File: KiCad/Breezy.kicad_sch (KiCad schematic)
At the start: 18 parts, among them J1 Line Voltage Input 120VAC / 6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, J2 Line Voltage Output 120VAC / 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, K1 5V, Q1 2N3904

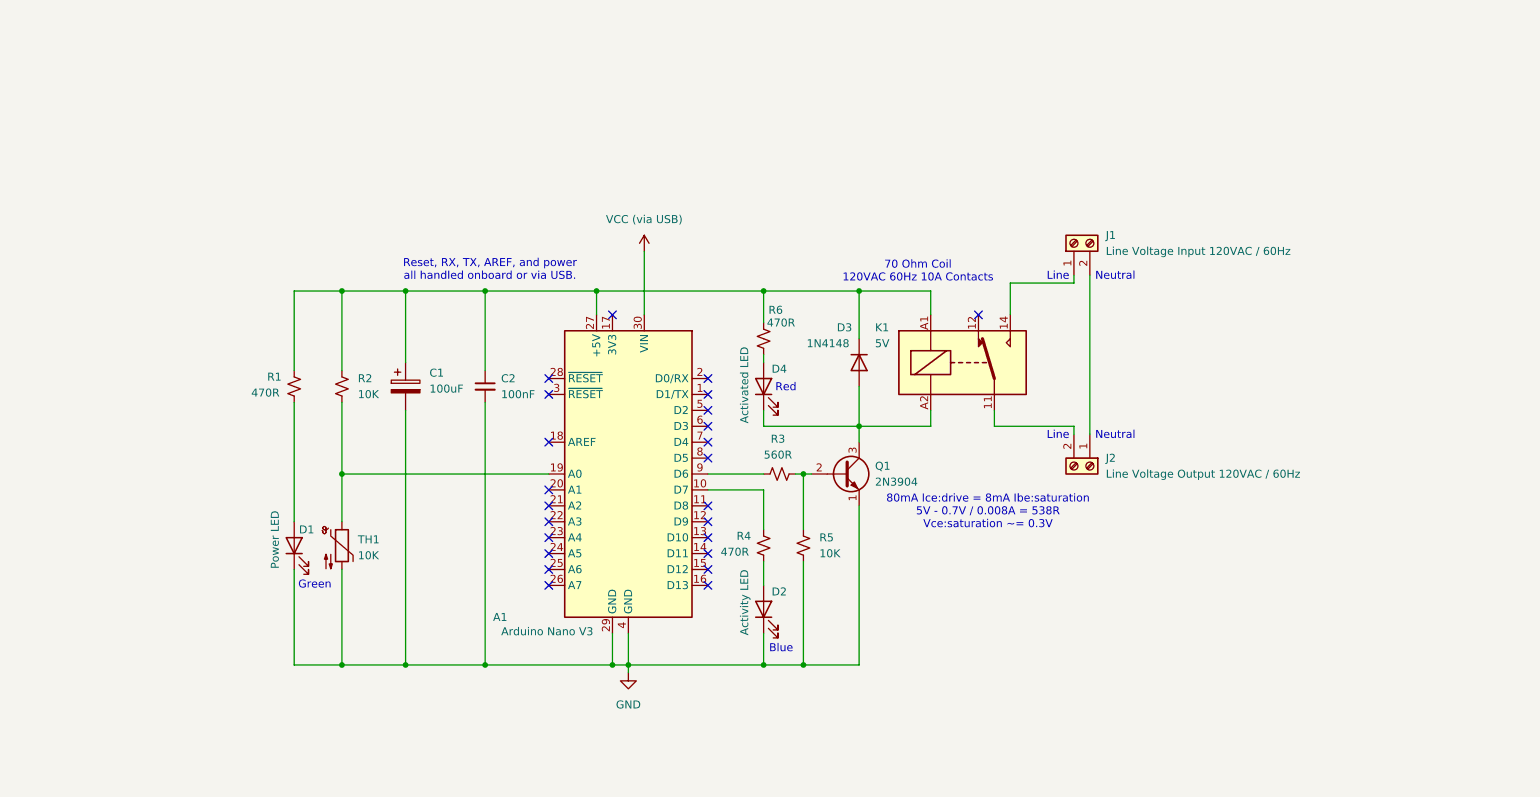
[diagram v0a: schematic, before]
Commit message: Update Breezy
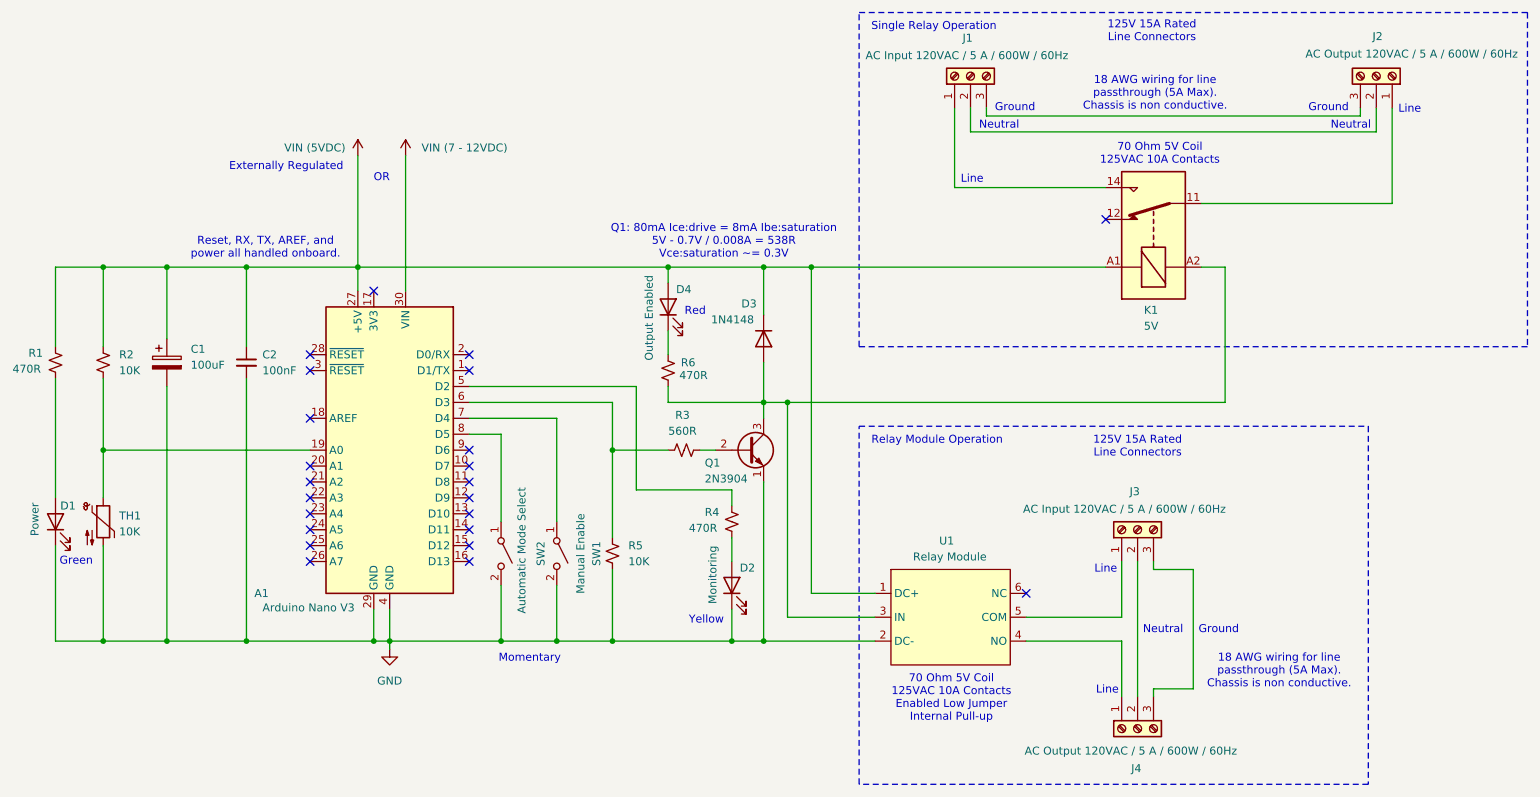
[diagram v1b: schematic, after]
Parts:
- removed J1: Line Voltage Input 120VAC / 60Hz, symbol Connector:Screw_Terminal_01x02
- removed J2: Line Voltage Output 120VAC / 60Hz, symbol Connector:Screw_Terminal_01x02
- added J1, J3: AC Input 120VAC / 5 A / 600W / 60Hz, symbol Connector:Screw_Terminal_01x03
- added J2, J4: AC Output 120VAC / 5 A / 600W / 60Hz, symbol Connector:Screw_Terminal_01x03
- added SW1: Manual Enable, symbol Switch:SW_SPST
- added SW2: Automatic Mode Select, symbol Switch:SW_SPST
- added U1: ~, symbol Custom:Relay Module
- D1: value Power LED -> Power
- D2: value Activity LED -> Monitoring
- D4: value Activated LED -> Output Enabled
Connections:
- net GND: now also SW1.2 (B), SW2.2 (B), U1.2 (DC-)
- net VIN (5VDC): now reaches A1.27 (+5V), C1.1, C2.1, D3.1 (K), K1.A1, R1.1, R2.1
- net VIN (5VDC): now also D4.2 (A), U1.1 (DC+); no longer R6.1
- net at D3.2 (A), K1.A2, Q1.3 (C): now also R6.2, U1.3 (IN); no longer D4.1 (K)
- net at K1.11: now also J2.1 (Pin_1)
- net at Q1.2 (B), R3.1: no longer R5.1
- net at R3.2: now also A1.6 (D3), R5.1; no longer A1.9 (D6)
- net at R4.1: now also A1.5 (D2); no longer A1.10 (D7)
- net at A1.7 (D4): now also SW1.1 (A)
- net at A1.8 (D5): now also SW2.1 (A)
- net at K1.14: now also J1.1 (Pin_1)
- net VCC (via USB) renamed VIN (7 - 12VDC)
- new net: J4.1 (Pin_1), U1.4 (NO)
- new net: J3.1 (Pin_1), U1.5 (COM)
- new net: D4.1 (K), R6.1
- new net: J3.2 (Pin_2), J4.2 (Pin_2)
- new net: J3.3 (Pin_3), J4.3 (Pin_3)
- new net: J1.2 (Pin_2), J2.2 (Pin_2)
- new net: J1.3 (Pin_3), J2.3 (Pin_3)
- no-connect marks 24 -> 23
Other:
- note added: "125V 15A Rated Line Connectors"
- note added: "18 AWG wiring for line passthrough (5A Max). Chassis is non conductive."
- note added: "70 Ohm 5V Coil 125VAC 10A Contacts"
- note added: "70 Ohm 5V Coil 125VAC 10A Contacts Enabled Low Jumper Internal Pull-up"
- note added: "Externally Regulated"
- note added: "Ground"
- note added: "Momentary"
- note added: "OR"
- note added: "Q1: 80mA Ice:drive = 8mA Ibe:saturation 5V - 0.7V / 0.008A = 538R Vce:saturation ~= 0.3V"
- note added: "Relay Module Operation"
- note added: "Reset, RX, TX, AREF, and power all handled onboard."
- note added: "Single Relay Operation"
- note added: "Yellow"
- note removed: "70 Ohm Coil 120VAC 60Hz 10A Contacts"
- note removed: "80mA Ice:drive = 8mA Ibe:saturation 5V - 0.7V / 0.008A = 538R Vce:saturation ~= 0.3V"
- note removed: "Blue"
- note removed: "Reset, RX, TX, AREF, and power all handled onboard or via USB."
- moved on the sheet: A1, C1, C2, D1, D2, D3, D4, K1, Q1, R1, R2, R3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
